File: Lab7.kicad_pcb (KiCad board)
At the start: 2 copper layers, 63.5 x 63.5 mm, 0 parts

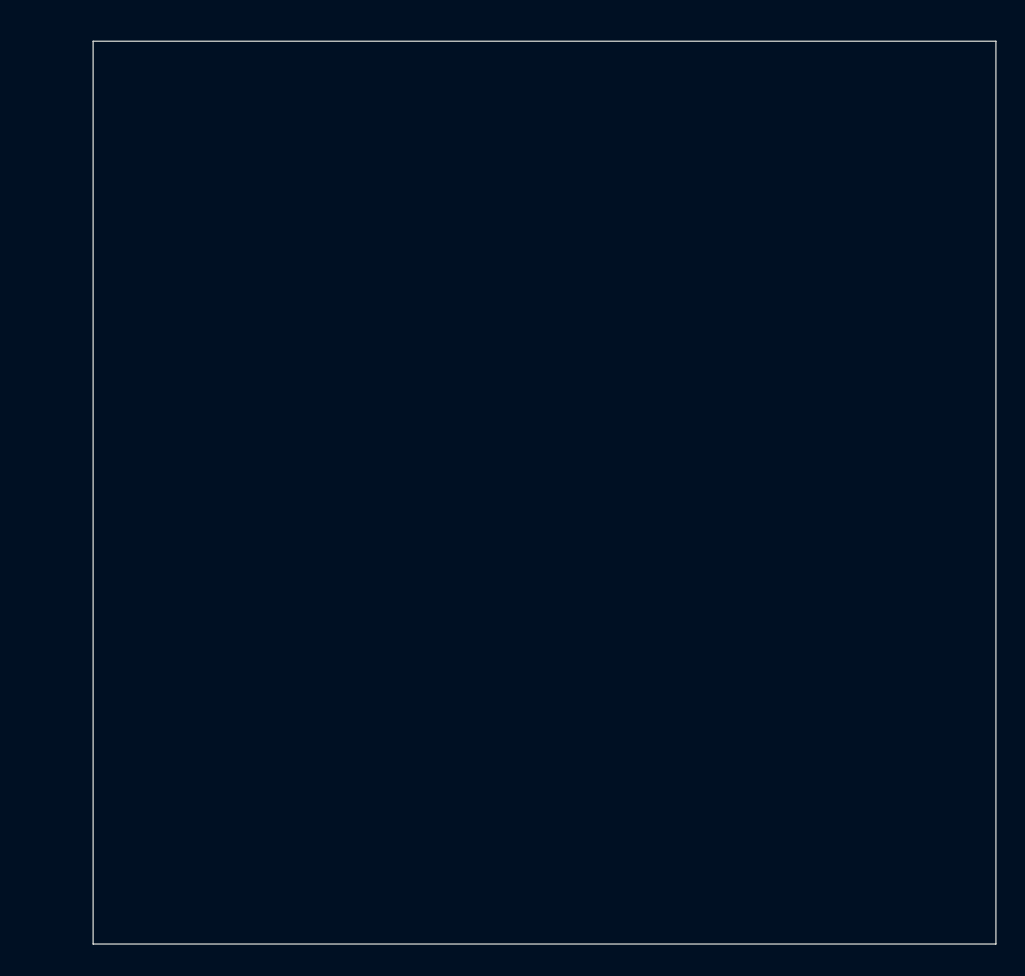
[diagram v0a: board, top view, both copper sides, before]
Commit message: gang
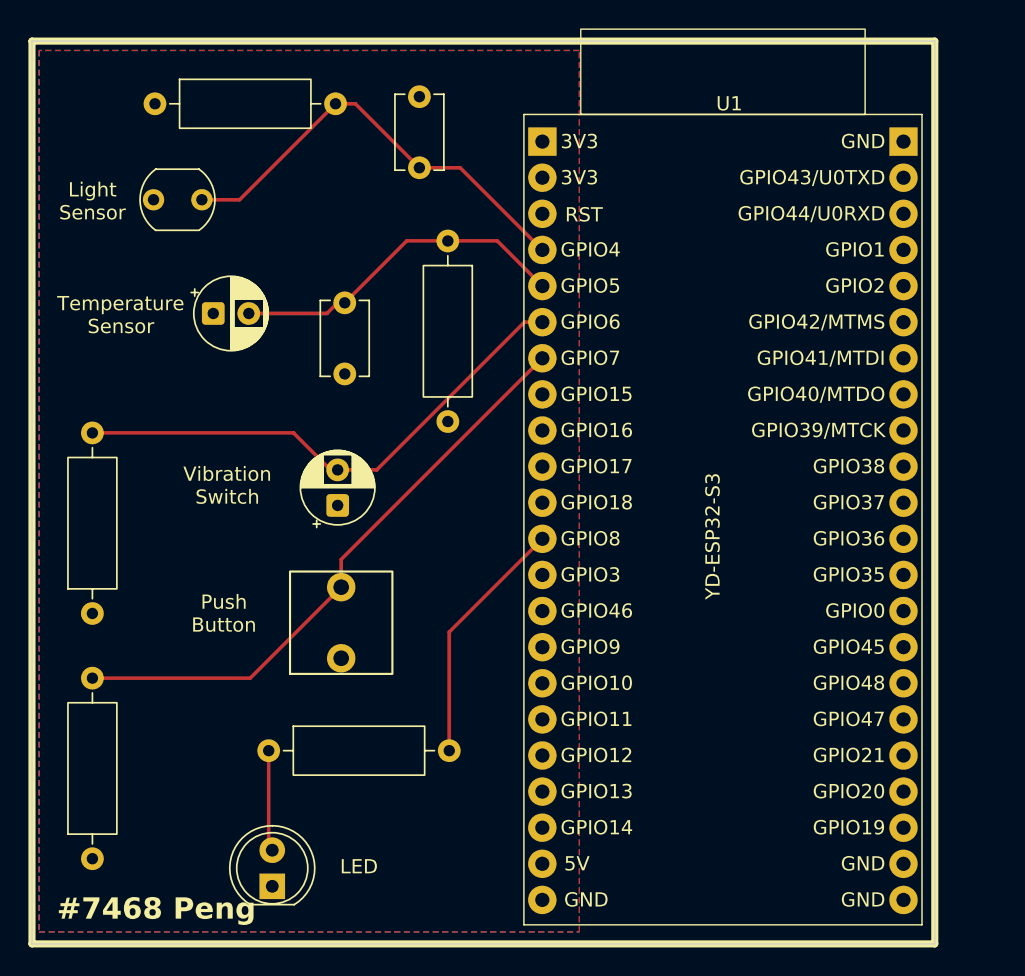
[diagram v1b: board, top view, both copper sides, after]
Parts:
- added C1: 100nF, Capacitor_THT:C_Disc_D5.1mm_W3.2mm_P5.00mm, F.Cu at (137.2, 78.8)
- added C2: 100nF, Capacitor_THT:C_Disc_D5.1mm_W3.2mm_P5.00mm, F.Cu at (132.0, 93.2)
- added D1: LED, LED_THT:LED_D5.0mm, F.Cu at (126.9, 129.3)
- added R1: 10k, Resistor_THT:R_Axial_DIN0309_L9.0mm_D3.2mm_P12.70mm_Horizontal, F.Cu at (118.7, 74.2)
- added R2: 10k, Resistor_THT:R_Axial_DIN0309_L9.0mm_D3.2mm_P12.70mm_Horizontal, F.Cu at (139.2, 83.9)
- added R3: 10k, Resistor_THT:R_Axial_DIN0309_L9.0mm_D3.2mm_P12.70mm_Horizontal, F.Cu at (114.2, 110.1)
- added R4: 10k, Resistor_THT:R_Axial_DIN0309_L9.0mm_D3.2mm_P12.70mm_Horizontal, F.Cu at (114.2, 127.3)
- added R5: 1k, Resistor_THT:R_Axial_DIN0309_L9.0mm_D3.2mm_P12.70mm_Horizontal, F.Cu at (126.7, 119.8)
- added R6: LDR07, OptoDevice:R_LDR_5.1x4.3mm_P3.4mm_Vertical, F.Cu at (118.5, 81.0)
- added SW1: Vibration Switch, Capacitor_THT:CP_Radial_D5.0mm_P2.50mm, F.Cu at (131.5, 102.5)
- added SW2: Push Button, SW_PUSH_6mm_2pin:SW_PUSH_6mm_2pin, F.Cu at (131.8, 110.8)
- added TH1: Thermistor_NTC, Capacitor_THT:CP_Radial_D5.0mm_P2.50mm, F.Cu at (122.8, 89.0)
- added U1: YD-ESP32-S3, YD-ESP32-S3:YD-ESP32-S3, F.Cu at (144.6, 75.0)
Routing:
- net Net-(U1-GPIO7): track 0.00 -> 42.1 mm
- net Net-(U1-GPIO6): track 0.00 -> 37.0 mm
- net Net-(U1-GPIO4): track 0.00 -> 31.0 mm
- net Net-(U1-GPIO5): track 0.00 -> 24.1 mm
- net Net-(U1-GPIO8): track 0.00 -> 17.6 mm
- net Net-(D1-A): track 0.00 -> 7.10 mm
- added copper zone on F.Cu, net /3.3V
- added copper zone on B.Cu, net GND
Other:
- board text added: "#7468 Peng"
- board text added: "LED"
- board text added: "Light Sensor"
- board text added: "Push Button"
- board text added: "Temperature Sensor"
- board text added: "Vibration Switch"
